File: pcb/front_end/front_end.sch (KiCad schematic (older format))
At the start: 43 parts, among them J1 SMA, J10 SMA, J11 SMA, J12 SMA, J13 SMA, J14 SMA, J15 SMA, J16 SMA, J17 SMA, J18 SMA, J19 SMA, J2 SMA, J20 SMA, J21 SMA, J22 SMA, J23 SMA, J24 SMA, J25 SMA, J26 SMA, J27 SMA, J28 SMA, J29 SMA, J3 SMA, J30 SMA, J31 SMA, J4 SMA, J5 SMA, J6 SMA, J7 SMP, J8 SMP, J9 SMA

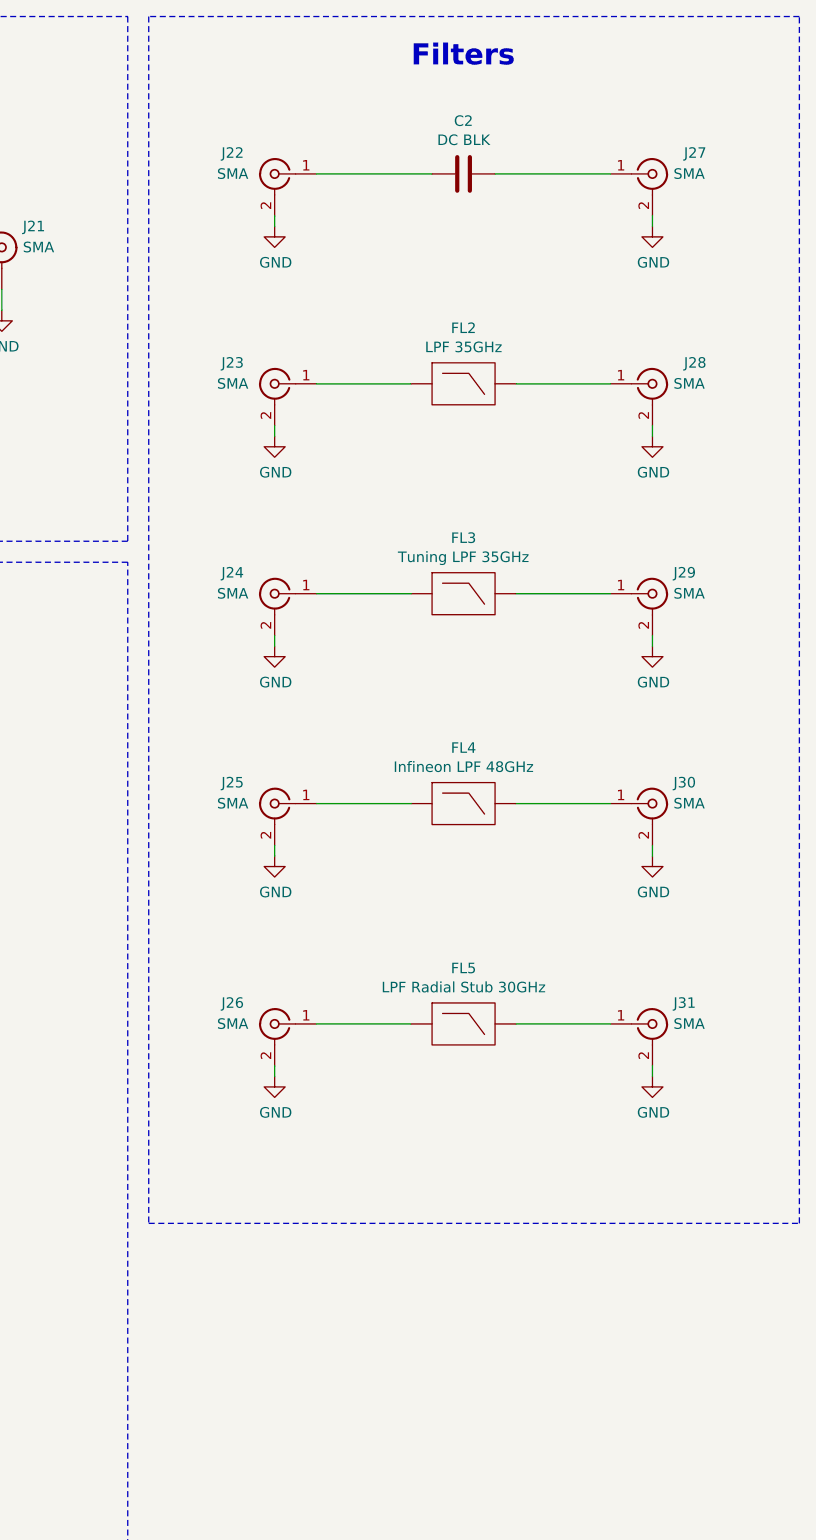
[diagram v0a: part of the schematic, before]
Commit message: Generated Fabrication files
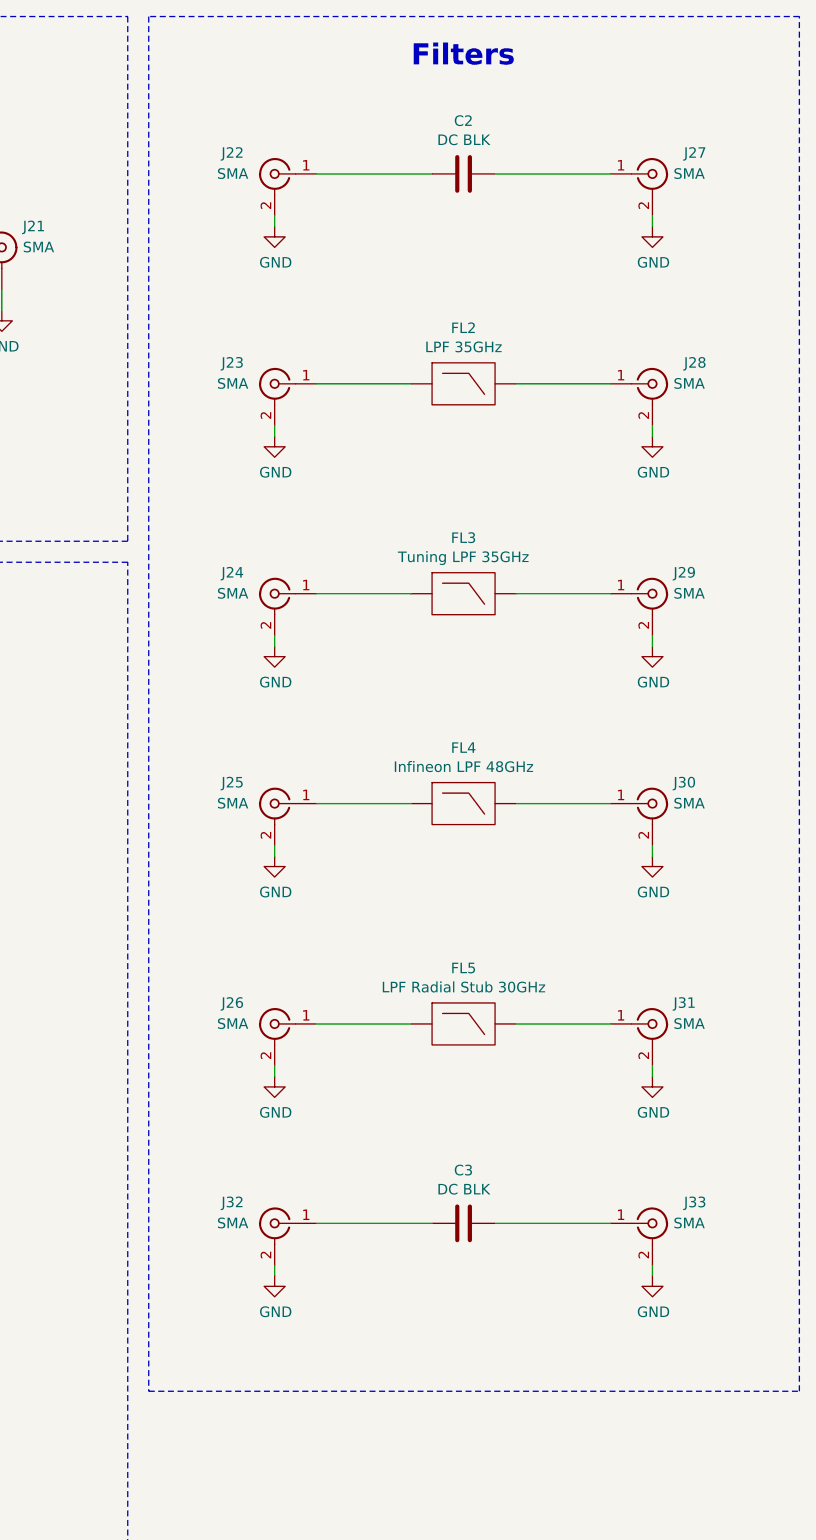
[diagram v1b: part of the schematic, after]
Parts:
- added C3: DC BLK, Capacitor_SMD:C_0402_1005Metric, symbol Device:C
- added J32, J33: SMA, bloop:292-06A-5, symbol Connector:Conn_Coaxial
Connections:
- net GND: now also J32.2 (Ext), J33.2 (Ext)
- new net: C3.1, J33.1 (In)
- new net: C3.2, J32.1 (In)
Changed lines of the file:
@@
 	14150 4700 14150 4750
 Wire Notes Line
-	11750 750  11750 6500
-Wire Notes Line
-	14850 6500 14850 750
+	11750 750  11750 7300
+Wire Notes Line
+	14850 7300 14850 750
 Wire Notes Line
 	14850 750  11750 750
@@
 SMP Bullet and TL Stub
 Wire Notes Line
-	11750 6500 14850 6500
+	11750 7300 14850 7300
 $Comp
 L Connector:Conn_Coaxial J31
@@
 Wire Wire Line
 	10150 1850 10850 1850
+Wire Wire Line
+	14150 6700 14150 6750
+$Comp
+L power:GND #PWR?
+U 1 1 5D80B028
+P 14150 6750
+F 0 "#PWR?" H 14150 6500 50  0001 C CNN
+F 1 "GND" H 14155 6577 50  0000 C CNN
+F 2 "" H 14150 6750 50  0001 C CNN
+F 3 "" H 14150 6750 50  0001 C CNN
+	1    14150 6750
+	1    0    0    -1
+$EndComp
+Wire Wire Line
+	13400 6500 13950 6500
+$Comp
+L power:GND #PWR?
+U 1 1 5D80B02F
+P 12350 6750
+F 0 "#PWR?" H 12350 6500 50  0001 C CNN
+F 1 "GND" H 12355 6577 50  0000 C CNN
+F 2 "" H 12350 6750 50  0001 C CNN
+F 3 "" H 12350 6750 50  0001 C CNN
+	1    12350 6750
+	1    0    0    -1
+$EndComp
+Wire Wire Line
+	12350 6700 12350 6750
+Wire Wire Line
+	13100 6500 12550 6500
+$Comp
+L Connector:Conn_Coaxial J33
+U 1 1 5D80B038
+P 14150 6500
+F 0 "J33" H 14300 6600 50  0000 L CNN
+F 1 "SMA" H 14250 6500 50  0000 L CNN
+F 2 "bloop:292-06A-5" H 14150 6500 50  0001 C CNN
+F 3 "https://www.hasco-inc.com/content/Southwest/End%20Launch/Jack/SMA_jack_endlaunch_genoutline.pdf" H 14150 6500 50  0001 C CNN
+F 4 "292-06A-5" H 14150 6500 50  0001 C CNN "MPN"
+	1    14150 6500
+	1    0    0    -1
+$EndComp
+$Comp
+L Connector:Conn_Coaxial J32
+U 1 1 5D80B03F
+P 12350 6500
+F 0 "J32" H 12550 6600 50  0000 C CNN
+F 1 "SMA" H 12550 6500 50  0000 C CNN
+F 2 "bloop:292-06A-5" H 12350 6500 50  0001 C CNN
+F 3 "https://www.hasco-inc.com/content/Southwest/End%20Launch/Jack/SMA_jack_endlaunch_genoutline.pdf" H 12350 6500 50  0001 C CNN
+F 4 "292-06A-5" H 12350 6500 50  0001 C CNN "MPN"
+	1    12350 6500
+	-1   0    0    -1
+$EndComp
+$Comp
+L Device:C C3
+U 1 1 5D80B045
+P 13250 6500
+F 0 "C3" V 12998 6500 50  0000 C CNN
+F 1 "DC BLK" V 13089 6500 50  0000 C CNN
+F 2 "Capacitor_SMD:C_0402_1005Metric" H 13288 6350 50  0001 C CNN
+F 3 "~" H 13250 6500 50  0001 C CNN
+	1    13250 6500
+	0    1    1    0
+$EndComp
 $EndSCHEMATC
